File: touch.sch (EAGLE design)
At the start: 37 parts, among them IC1 MAX203ECWP, IC2 PIC18F14Q41-I_SO

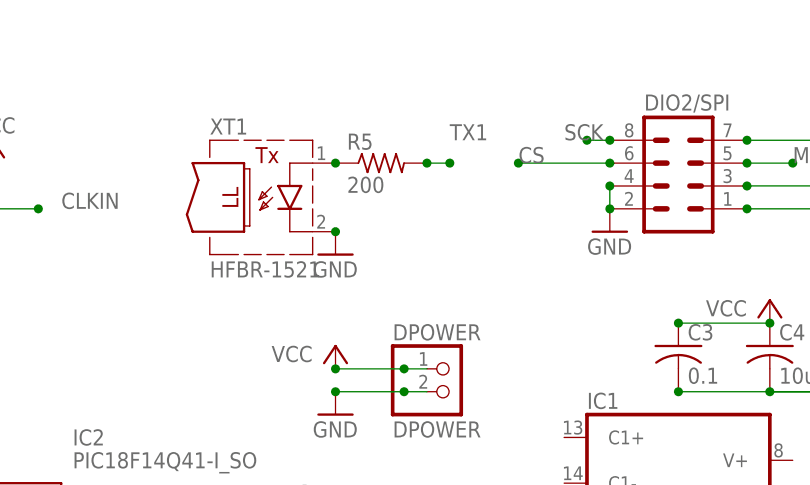
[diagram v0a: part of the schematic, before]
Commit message: up
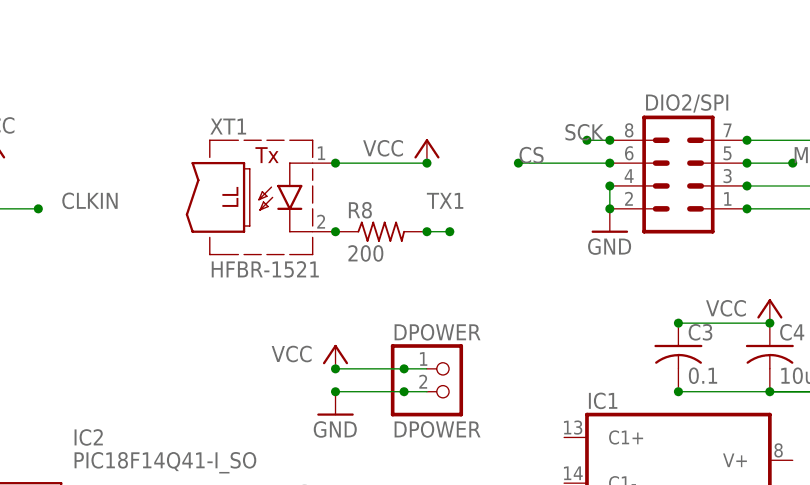
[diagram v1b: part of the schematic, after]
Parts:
- removed R5: 200, rcl:R-US_R0805
- added R8: 200, rcl:R-US_R0805
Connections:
- removed net N$19: R5.1, XT1.A
- new net N$10: R8.1, XT1.C
- net GND: no longer XT1.C
- net TX1: now also R8.2; no longer R5.2
- net VCC: now also XT1.A
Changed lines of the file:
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@@
 <?xml version="1.0" encoding="utf-8"?>
 <!DOCTYPE eagle SYSTEM "eagle.dtd">
-<eagle version="9.7.0">
+<eagle version="9.6.2">
 <drawing>
 <settings>
@@
 <part name="GND16" library="supply1" library_urn="urn:adsk.eagle:library:371" deviceset="GND" device=""/>
 <part name="R4" library="rcl" library_urn="urn:adsk.eagle:library:334" deviceset="R-US_" device="R0805" package3d_urn="urn:adsk.eagle:package:23553/2" value="1.2k"/>
-<part name="R5" library="rcl" library_urn="urn:adsk.eagle:library:334" deviceset="R-US_" device="R0805" package3d_urn="urn:adsk.eagle:package:23553/2" value="200"/>
-<part name="GND17" library="supply1" library_urn="urn:adsk.eagle:library:371" deviceset="GND" device=""/>
 <part name="C7" library="rcl" library_urn="urn:adsk.eagle:library:334" deviceset="C-US" device="C0805" package3d_urn="urn:adsk.eagle:package:23617/2" value="10uf"/>
 <part name="GND18" library="supply1" library_urn="urn:adsk.eagle:library:371" deviceset="GND" device=""/>
@@
 <part name="GND7" library="supply1" library_urn="urn:adsk.eagle:library:371" deviceset="GND" device=""/>
 <part name="P+12" library="supply1" library_urn="urn:adsk.eagle:library:371" deviceset="VCC" device=""/>
+<part name="R8" library="rcl" library_urn="urn:adsk.eagle:library:334" deviceset="R-US_" device="R0805" package3d_urn="urn:adsk.eagle:package:23553/2" value="200"/>
+<part name="P+13" library="supply1" library_urn="urn:adsk.eagle:library:371" deviceset="VCC" device=""/>
 </parts>
 <sheets>
@@
 <attribute name="VALUE" x="13.97" y="-13.462" size="1.778" layer="96"/>
 </instance>
-<instance part="R5" gate="G$1" x="96.52" y="91.44" smashed="yes">
-<attribute name="NAME" x="92.71" y="92.9386" size="1.778" layer="95"/>
-<attribute name="VALUE" x="92.71" y="88.138" size="1.778" layer="96"/>
-</instance>
-<instance part="GND17" gate="1" x="91.44" y="81.28" smashed="yes">
-<attribute name="VALUE" x="88.9" y="78.74" size="1.778" layer="96"/>
-</instance>
 <instance part="C7" gate="G$1" x="99.06" y="-7.62" smashed="yes">
 <attribute name="NAME" x="100.076" y="-6.985" size="1.778" layer="95"/>
@@
 <instance part="P+12" gate="VCC" x="91.44" y="71.12" smashed="yes">
 <attribute name="VALUE" x="88.9" y="71.12" size="1.778" layer="96" rot="R180"/>
+</instance>
+<instance part="R8" gate="G$1" x="96.52" y="83.82" smashed="yes">
+<attribute name="NAME" x="92.71" y="85.3186" size="1.778" layer="95"/>
+<attribute name="VALUE" x="92.71" y="80.518" size="1.778" layer="96"/>
+</instance>
+<instance part="P+13" gate="VCC" x="101.6" y="93.98" smashed="yes">
+<attribute name="VALUE" x="99.06" y="93.98" size="1.778" layer="96" rot="R180"/>
 </instance>
 </instances>
@@
 <pinref part="GND16" gate="1" pin="GND"/>
 <junction x="0" y="5.08"/>
-</segment>
-<segment>
-<pinref part="XT1" gate="A" pin="C"/>
-<pinref part="GND17" gate="1" pin="GND"/>
-<junction x="91.44" y="83.82"/>
 </segment>
 <segment>
@@
 <wire x1="99.06" y1="68.58" x2="91.44" y2="68.58" width="0.1524" layer="91"/>
 <junction x="91.44" y="68.58"/>
+</segment>
+<segment>
+<pinref part="XT1" gate="A" pin="A"/>
+<pinref part="P+13" gate="VCC" pin="VCC"/>
+<wire x1="101.6" y1="91.44" x2="91.44" y2="91.44" width="0.1524" layer="91"/>
+<junction x="91.44" y="91.44"/>
+<junction x="101.6" y="91.44"/>
 </segment>
 </net>
@@
 </segment>
 <segment>
-<wire x1="104.14" y1="91.44" x2="101.6" y2="91.44" width="0.1524" layer="91"/>
-<pinref part="R5" gate="G$1" pin="2"/>
-<label x="104.14" y="93.98" size="1.778" layer="95"/>
-<junction x="101.6" y="91.44"/>
-<junction x="104.14" y="91.44"/>
-</segment>
-<segment>
 <wire x1="104.14" y1="10.16" x2="101.6" y2="10.16" width="0.1524" layer="91"/>
 <pinref part="TTLRS232" gate="G$1" pin="3"/>
@@
 <junction x="104.14" y="10.16"/>
 <label x="104.14" y="10.16" size="1.778" layer="95"/>
+</segment>
+<segment>
+<wire x1="104.14" y1="83.82" x2="101.6" y2="83.82" width="0.1524" layer="91"/>
+<pinref part="R8" gate="G$1" pin="2"/>
+<junction x="101.6" y="83.82"/>
+<junction x="104.14" y="83.82"/>
+<label x="101.6" y="86.36" size="1.778" layer="95"/>
 </segment>
 </net>
@@
 </segment>
 </net>
-<net name="N$19" class="0">
-<segment>
-<pinref part="XT1" gate="A" pin="A"/>
-<pinref part="R5" gate="G$1" pin="1"/>
-<junction x="91.44" y="91.44"/>
-</segment>
-</net>
 <net name="N$16" class="1">
 <segment>
@@
 </segment>
 </net>
+<net name="N$10" class="0">
+<segment>
+<pinref part="XT1" gate="A" pin="C"/>
+<pinref part="R8" gate="G$1" pin="1"/>
+<junction x="91.44" y="83.82"/>
+</segment>
+</net>
